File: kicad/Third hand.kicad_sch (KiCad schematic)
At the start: 66 parts, among them U301 74HC595, U302 74HC595

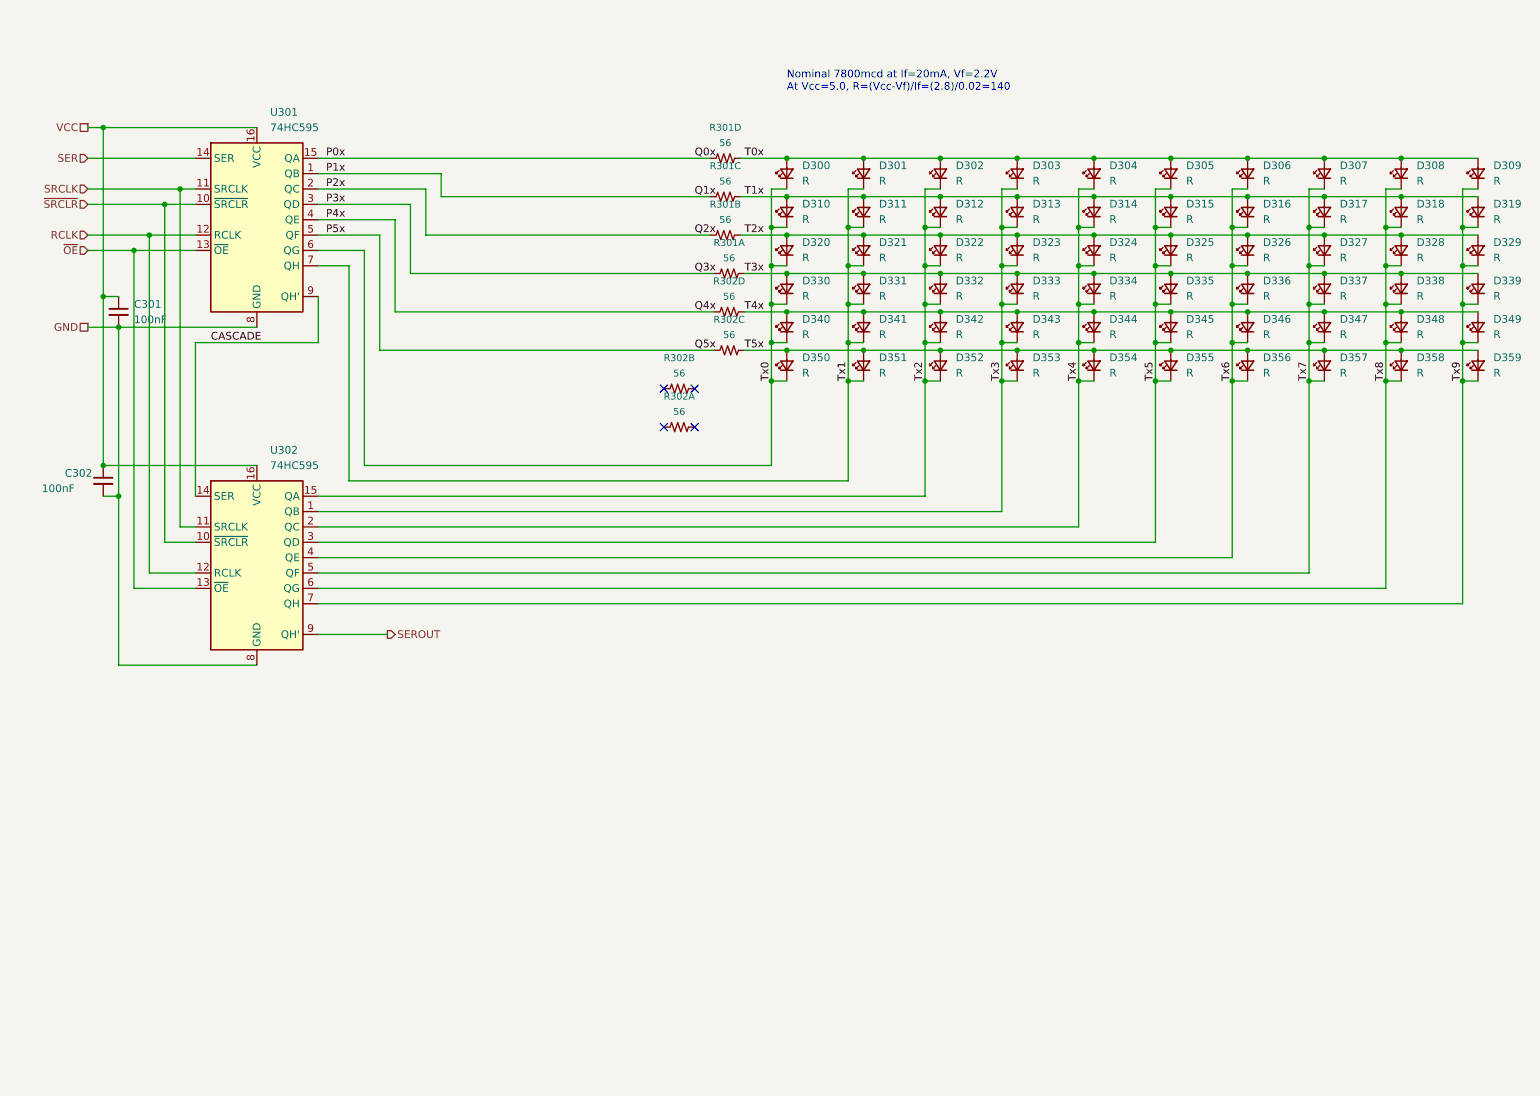
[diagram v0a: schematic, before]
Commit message: Matrix8x8 stuff
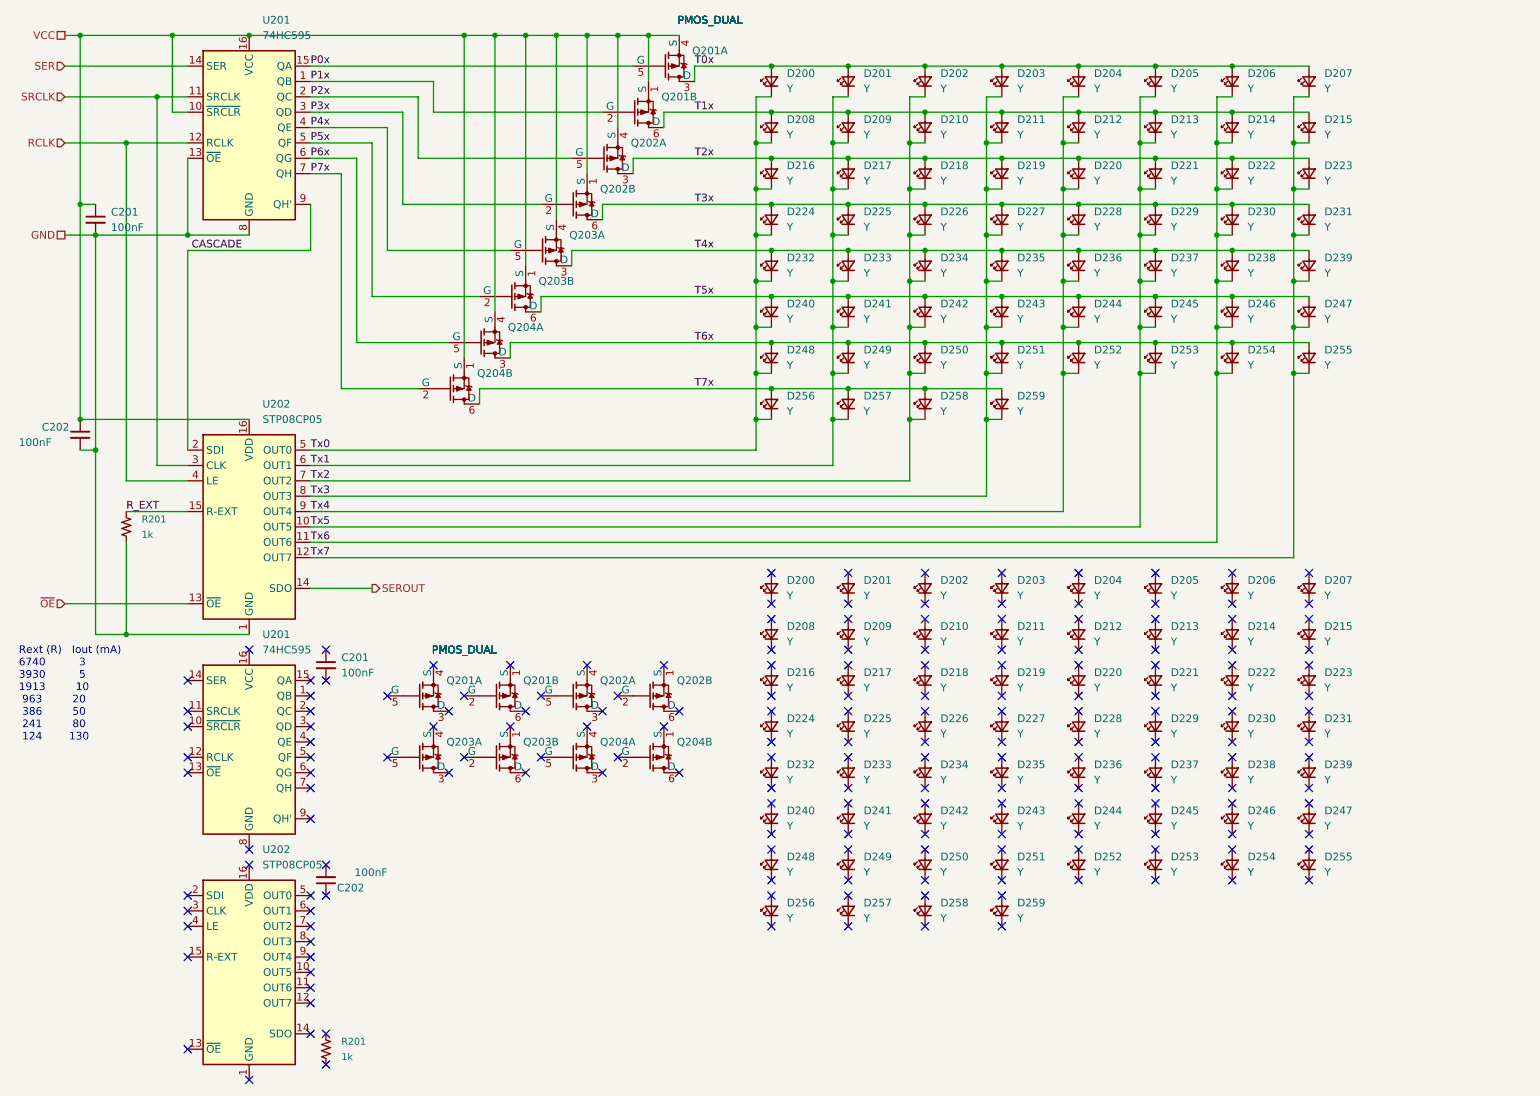
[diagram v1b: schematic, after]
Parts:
- removed C301, C302: 100nF, Capacitor_SMD:C_0603_1608Metric, symbol Device:C_Small
- removed D300, D301, D302, D303, D304, D305, D306, D307, D308, D309, D310, D311, D312, D313, D314, D315, D316, D317, D318, D319, D320, D321, D322, D323, D324, D325, D326, D327, D328, D329, D330, D331, D332, D333, D334, D335, D336, D337, D338, D339, D340, D341, D342, D343, D344, D345, D346, D347, D348, D349, D350, D351, D352, D353, D354, D355, D356, D357, D358, D359: R, KwanSystems:D_KINGBRIGHT_DOME, symbol Device:LED_Small
- removed R301, R302: 56, KwanSystems:R_Array_Convex_4x0402, symbol KwanSystems:RP4
- removed U301, U302: 74HC595, Package_SO:TSSOP-16_4.4x5mm_P0.65mm, symbol 74xx:74HC595
- added C201 (x2), C202 (x2): 100nF, Capacitor_SMD:C_0603_1608Metric, symbol Device:C_Small
- added D200 (x2), D201 (x2), D202 (x2), D203 (x2), D204 (x2), D205 (x2), D206 (x2), D207 (x2), D208 (x2), D209 (x2), D210 (x2), D211 (x2), D212 (x2), D213 (x2), D214 (x2), D215 (x2), D216 (x2), D217 (x2), D218 (x2), D219 (x2), D220 (x2), D221 (x2), D222 (x2), D223 (x2), D224 (x2), D225 (x2), D226 (x2), D227 (x2), D228 (x2), D229 (x2), D230 (x2), D231 (x2), D232 (x2), D233 (x2), D234 (x2), D235 (x2), D236 (x2), D237 (x2), D238 (x2), D239 (x2), D240 (x2), D241 (x2), D242 (x2), D243 (x2), D244 (x2), D245 (x2), D246 (x2), D247 (x2), D248 (x2), D249 (x2), D250 (x2), D251 (x2), D252 (x2), D253 (x2), D254 (x2), D255 (x2), D256 (x2), D257 (x2), D258 (x2), D259 (x2): Y, KwanSystems:D_KINGBRIGHT_DOME, symbol Device:LED_Small
- added Q201 (x2), Q202 (x2), Q203 (x2), Q204 (x2): PMOS_DUAL, Package_TO_SOT_SMD:SOT-363_SC-70-6, symbol KwanSystems:PMOS_DUAL
- added R201 (x2): 1k, Resistor_SMD:R_0603_1608Metric, symbol KwanSystems:RESISTOR
- added U201 (x2): 74HC595, Package_SO:TSSOP-16_4.4x5mm_P0.65mm, symbol 74xx:74HC595
- added U202 (x2): STP08CP05, Package_SO:TSSOP-16_4.4x5mm_P0.65mm, symbol Driver_LED:STP08CP05
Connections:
- net CASCADE: now also U201.9 (QH'), U202.2 (SDI)
- net GND: now also C201.2, C202.2, R201.1, U201.13 (~{OE}), U201.8 (GND), U202.1 (GND)
- net P0x: now also Q201.5 (G), U201.15 (QA)
- net P1x: now also Q201.2 (G), U201.1 (QB)
- net P2x: now also Q202.5 (G), U201.2 (QC)
- net P3x: now also Q202.2 (G), U201.3 (QD)
- net P4x: now also Q203.5 (G), U201.4 (QE)
- net P5x: now also Q203.2 (G), U201.5 (QF)
- net RCLK: now also U201.12 (RCLK), U202.4 (LE)
- net SER: now also U201.14 (SER)
- net SEROUT: now also U202.14 (SDO)
- net SRCLK: now also U201.11 (SRCLK), U202.3 (CLK)
- net T0x: now also D200.2 (A), D201.2 (A), D202.2 (A), D203.2 (A), D204.2 (A), D205.2 (A), D206.2 (A), D207.2 (A), Q201.3 (D)
- net T1x: now also D208.2 (A), D209.2 (A), D210.2 (A), D211.2 (A), D212.2 (A), D213.2 (A), D214.2 (A), D215.2 (A), Q201.6 (D)
- net T2x: now also D216.2 (A), D217.2 (A), D218.2 (A), D219.2 (A), D220.2 (A), D221.2 (A), D222.2 (A), D223.2 (A), Q202.3 (D)
- net T3x: now also D224.2 (A), D225.2 (A), D226.2 (A), D227.2 (A), D228.2 (A), D229.2 (A), D230.2 (A), D231.2 (A), Q202.6 (D)
- net T4x: now also D232.2 (A), D233.2 (A), D234.2 (A), D235.2 (A), D236.2 (A), D237.2 (A), D238.2 (A), D239.2 (A), Q203.3 (D)
- net T5x: now also D240.2 (A), D241.2 (A), D242.2 (A), D243.2 (A), D244.2 (A), D245.2 (A), D246.2 (A), D247.2 (A), Q203.6 (D)
- net Tx0: now also D200.1 (K), D208.1 (K), D216.1 (K), D224.1 (K), D232.1 (K), D240.1 (K), D248.1 (K), D256.1 (K), U202.5 (OUT0)
- net Tx1: now also D201.1 (K), D209.1 (K), D217.1 (K), D225.1 (K), D233.1 (K), D241.1 (K), D249.1 (K), D257.1 (K), U202.6 (OUT1)
- net Tx2: now also D202.1 (K), D210.1 (K), D218.1 (K), D226.1 (K), D234.1 (K), D242.1 (K), D250.1 (K), D258.1 (K), U202.7 (OUT2)
- net Tx3: now also D203.1 (K), D211.1 (K), D219.1 (K), D227.1 (K), D235.1 (K), D243.1 (K), D251.1 (K), D259.1 (K), U202.8 (OUT3)
- net Tx4: now also D204.1 (K), D212.1 (K), D220.1 (K), D228.1 (K), D236.1 (K), D244.1 (K), D252.1 (K), U202.9 (OUT4)
- net Tx5: now also D205.1 (K), D213.1 (K), D221.1 (K), D229.1 (K), D237.1 (K), D245.1 (K), D253.1 (K), U202.10 (OUT5)
- net Tx6: now also D206.1 (K), D214.1 (K), D222.1 (K), D230.1 (K), D238.1 (K), D246.1 (K), D254.1 (K), U202.11 (OUT6)
- net Tx7: now also D207.1 (K), D215.1 (K), D223.1 (K), D231.1 (K), D239.1 (K), D247.1 (K), D255.1 (K), U202.12 (OUT7)
- net VCC: now also C201.1, C202.1, Q201.1 (S), Q201.4 (S), Q202.1 (S), Q202.4 (S), Q203.1 (S), Q203.4 (S), Q204.1 (S), Q204.4 (S), U201.10 (~{SRCLR}), U201.16 (VCC), U202.16 (VDD)
- net ~{OE}: now also U202.13 (~{OE})
- new net P6x: Q204.5 (G), U201.6 (QG)
- new net P7x: Q204.2 (G), U201.7 (QH)
- new net R_EXT: R201.2, U202.15 (R-EXT)
- new net T6x: D248.2 (A), D249.2 (A), D250.2 (A), D251.2 (A), D252.2 (A), D253.2 (A), D254.2 (A), D255.2 (A), Q204.3 (D)
- new net T7x: D256.2 (A), D257.2 (A), D258.2 (A), D259.2 (A), Q204.6 (D)
- no-connect marks 4 -> 182
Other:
- note added: "Rext (R) Iout (mA) 6740 3 3930 5 1913 10 963 20 386 50 241 80 124 130"
- note removed: "Nominal 7800mcd at If=20mA, Vf=2.2V At Vcc=5.0, R=(Vcc-Vf)/If=(2.8)/0.02=140"
